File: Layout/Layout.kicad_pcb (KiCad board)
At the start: 2 copper layers, 70 x 50 mm, 73 parts, among them IC1 VL53L4CDV0DH_1, IC3 STM32F042G4U6, IC4 MAX4231AUT+T, J1 Conn_01x07_Pin, J2 USB_B_Micro, J3 Conn_01x03_Pin, J4 Conn_01x04_Pin, SW1 SW_Omron_B3FS, SW3 SW_Omron_B3FS, U1 INA197, U3 XC6210B332MR, U6 USBLC6-2SC6, Y1 SG-210STF_8.0000ML5

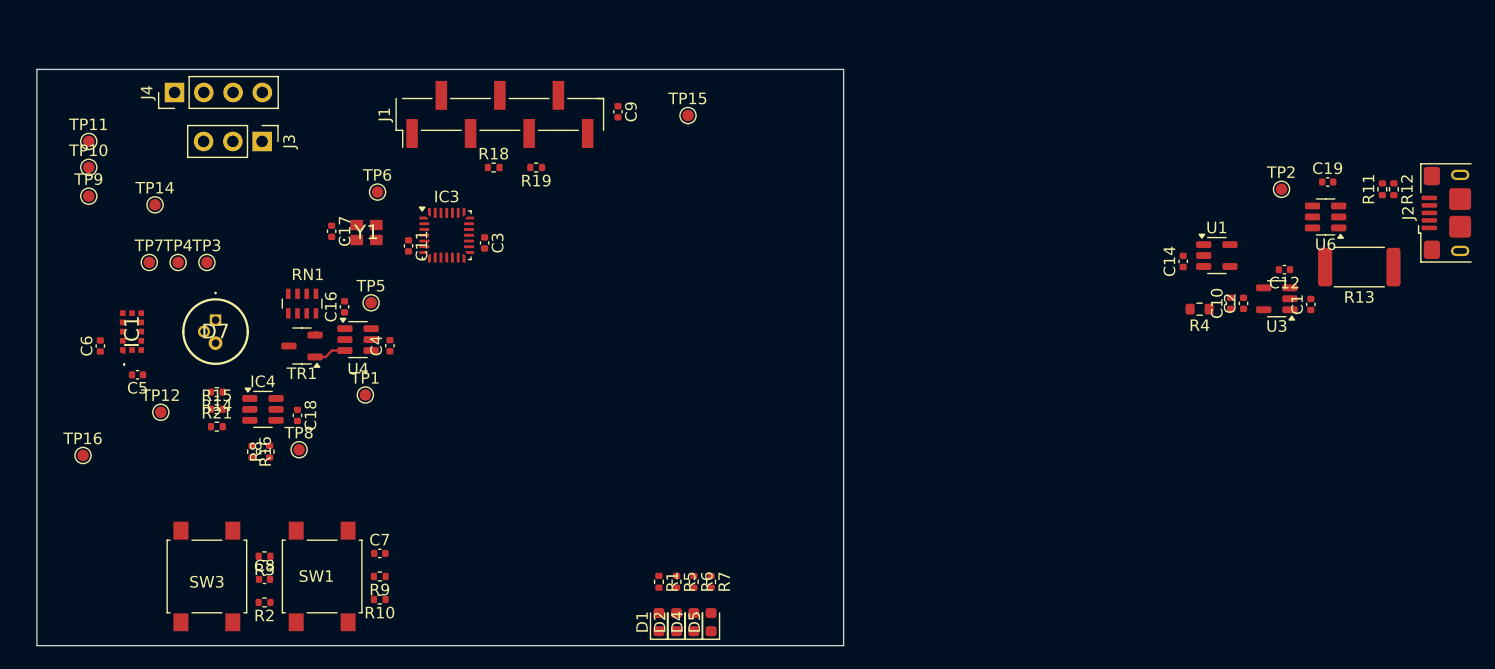
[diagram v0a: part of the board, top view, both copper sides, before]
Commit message: Compact version
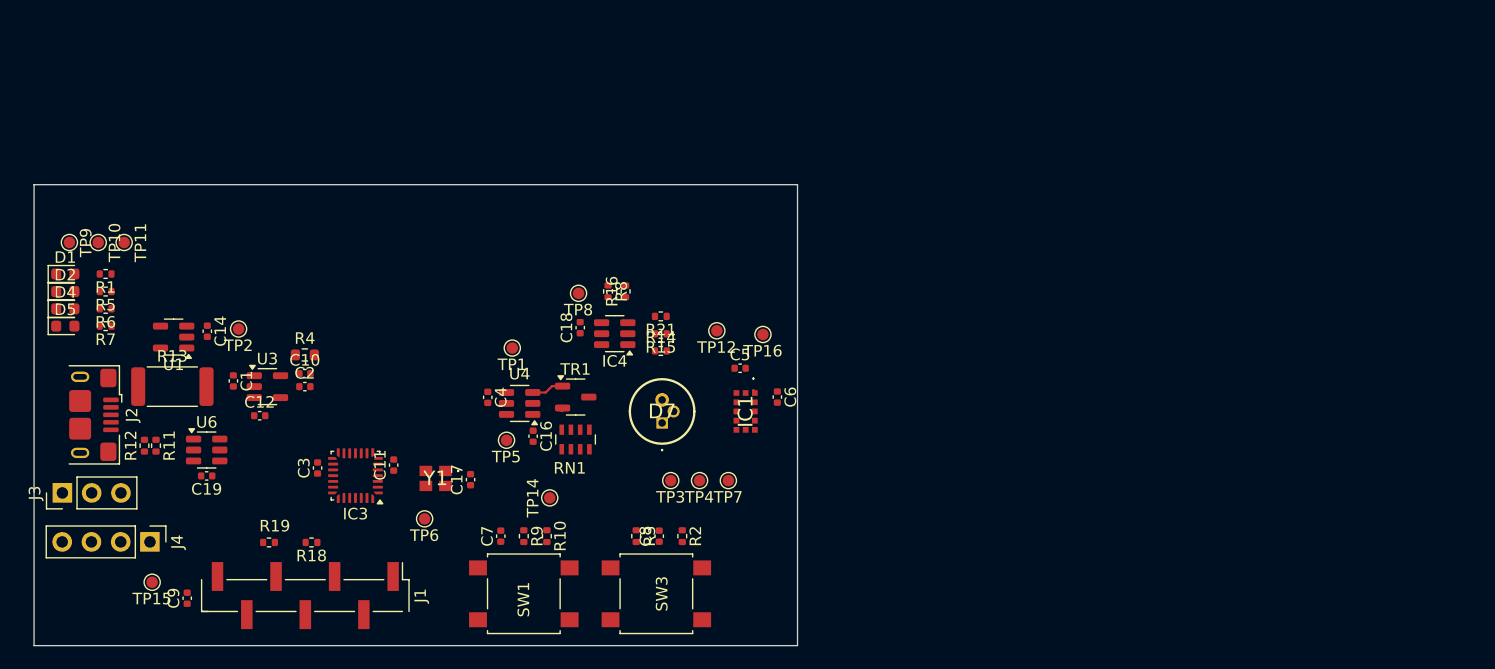
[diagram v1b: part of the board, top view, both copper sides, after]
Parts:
- moved J2 121.0 mm to (47.8, 99.0), turned to -90 degrees
- moved R12 110.7 mm to (53.3, 101.6), turned to 90 degrees
- moved R11 108.7 mm to (54.3, 101.6), turned to -90 degrees
- moved R13 103.5 mm to (55.8, 96.5), turned to 0 degrees
- moved C19 100.6 mm to (58.7, 104.3), turned to 180 degrees
- moved U6 99.2 mm to (58.7, 102.0), turned to 0 degrees
- moved C1 93.7 mm to (61.0, 96.0), turned to -90 degrees
- moved TP2 91.3 mm to (61.5, 91.5), turned to 180 degrees
- moved U1 90.8 mm to (55.9, 92.2), turned to 180 degrees
- moved C12 89.8 mm to (63.3, 99.0), turned to 0 degrees
- moved U3 87.9 mm to (64.0, 96.5), turned to 0 degrees
- moved C14 84.9 mm to (58.8, 91.7), turned to -90 degrees
- moved C2 81.8 mm to (67.2, 96.5), turned to 0 degrees
- moved C10 80.6 mm to (67.2, 95.4), turned to 0 degrees
- moved R4 77.7 mm to (67.2, 93.8), turned to 0 degrees
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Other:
- board size 70 x 50 mm -> 66.2 x 40 mm
